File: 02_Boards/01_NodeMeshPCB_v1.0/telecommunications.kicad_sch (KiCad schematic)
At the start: 4 parts, among them J3 SMAJPHRATH1, U10 LC76GABMD, U5 HT-RA62

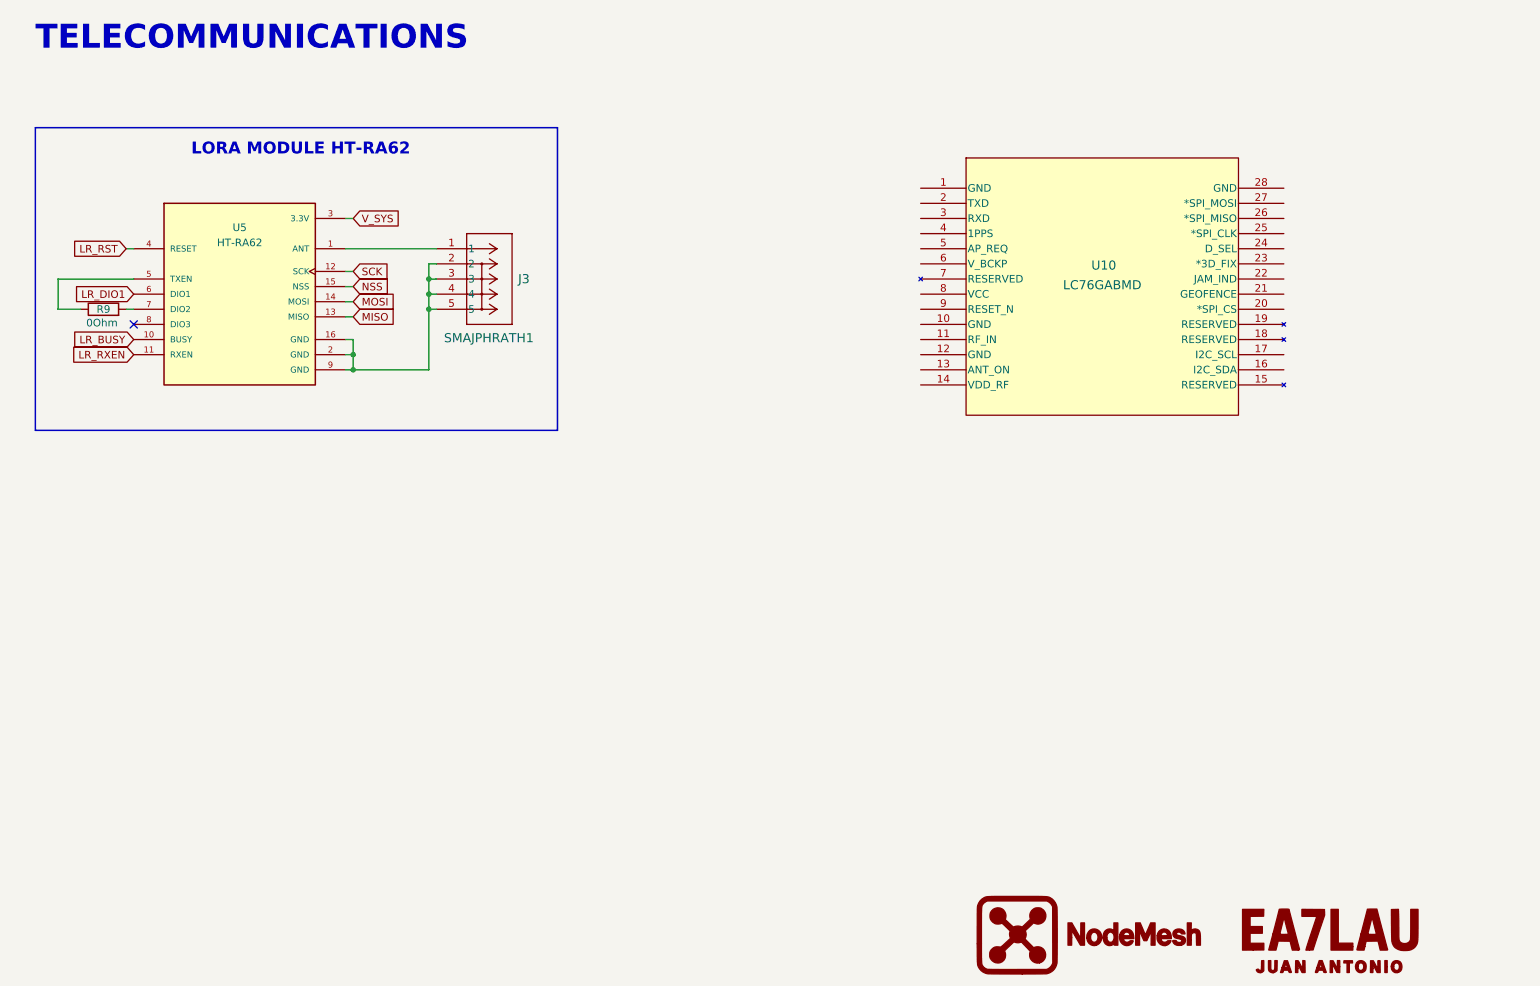
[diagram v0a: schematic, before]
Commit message: PCB placement
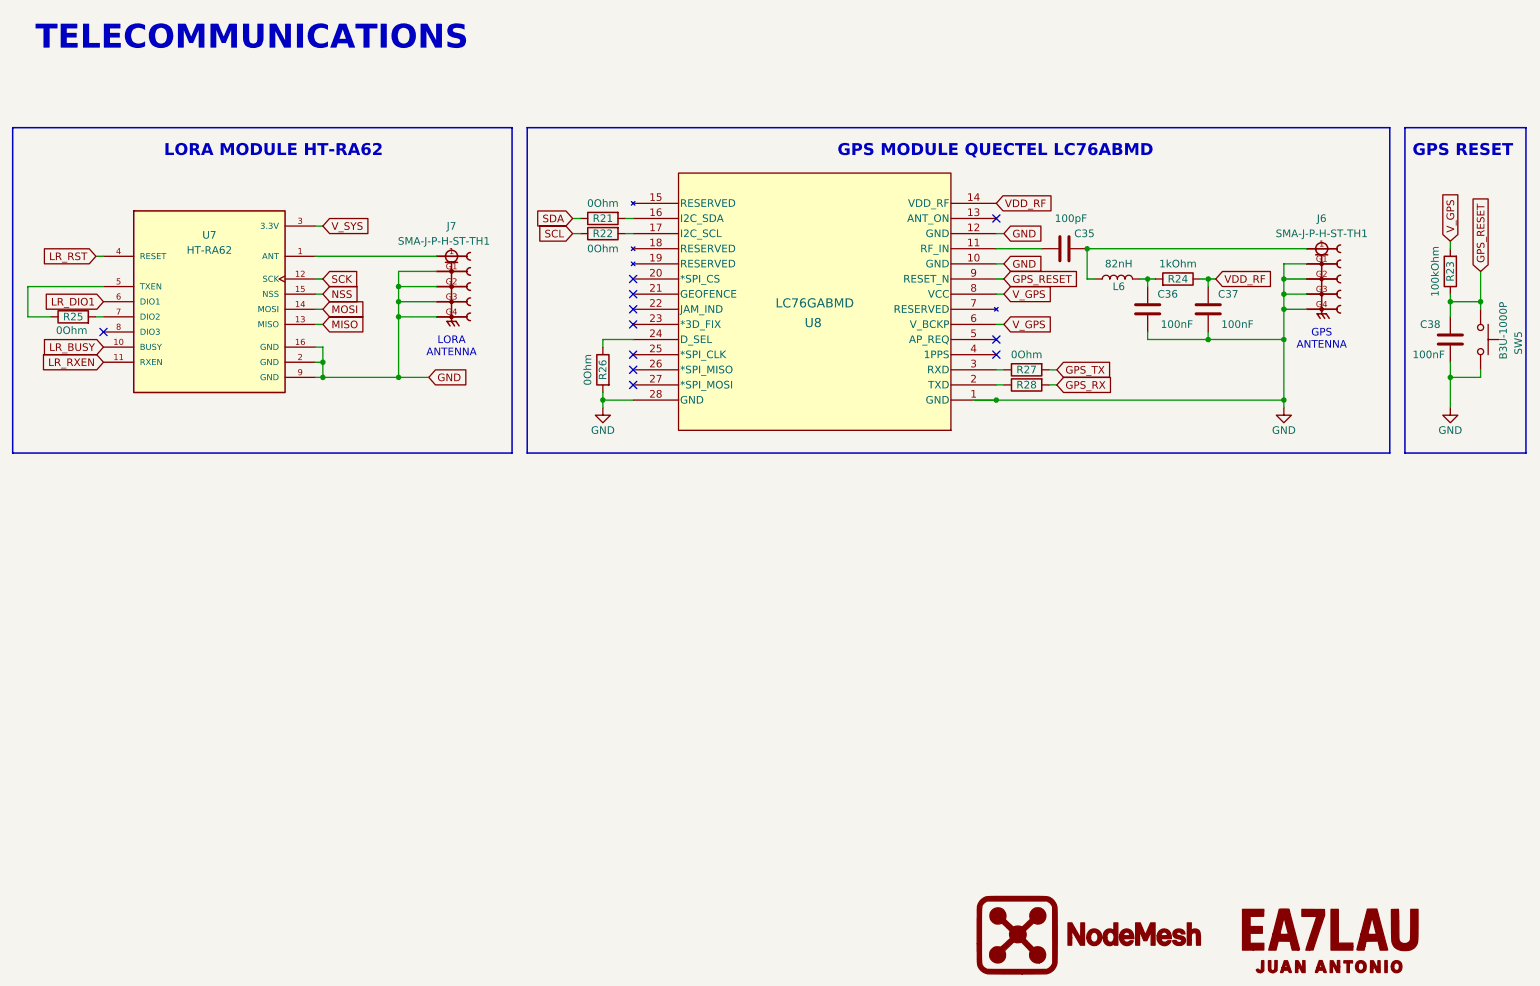
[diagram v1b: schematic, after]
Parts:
- removed J3: SMAJPHRATH1, CONN_SMA-J-P-H-RA-TH1_SAI, symbol SMAJPHRATH1:SMA-J-P-H-RA-TH1
- added C35: 100pF, Capacitor_SMD:C_0603_1608Metric, symbol Device:C
- added C36, C37, C38: 100nF, Capacitor_SMD:C_0603_1608Metric, symbol Device:C
- added J6, J7: SMA-J-P-H-ST-TH1, 01_Footprints:SMA-J-P-H-ST-TH1, symbol SMA-J-P-H-ST-TH1:SMA-J-P-H-ST-TH1
- added L6: 82nH, Inductor_SMD:L_0603_1608Metric, symbol Device:L
- added R21, R22, R26, R27, R28: 0Ohm, Resistor_SMD:R_0603_1608Metric, symbol Device:R
- added R23: 100kOhm, Resistor_SMD:R_0603_1608Metric, symbol Device:R
- added R24: 1kOhm, Resistor_SMD:R_0603_1608Metric, symbol Device:R
- added SW5: B3U-1000P, Button_Switch_SMD:SW_SPST_B3U-1000P, symbol Switch:SW_Push
- R25: renamed from R9; footprint (none) -> Resistor_SMD:R_0603_1608Metric
- U7: renamed from U5; footprint (none) -> 01_Footprints:HT-RA62
- U8: renamed from U10; footprint LC76G_QWS -> 01_Footprints:LC76GABMD
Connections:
- net GND: now reaches U8.1 (GND)
- net GND: now also U7.16 (GND), U7.2 (GND), U7.9 (GND), U8.10 (GND), U8.12 (GND), U8.28 (GND), C36.2, C37.2, C38.2, J6.G1, J6.G2, J6.G3, J6.G4, J7.G1, J7.G2, J7.G3, J7.G4, R26.2, SW5.2
- net at U8.11 (RF_IN): now also C35.1
- net VDD_RF: now reaches U8.14 (VDD_RF)
- net VDD_RF: now also C37.1, R24.1
- net at U8.16 (I2C_SDA): now also R21.2
- net at U8.17 (I2C_SCL): now also R22.2
- net at U8.2 (TXD): now also R28.1
- net at U8.24 (D_SEL): now also R26.1
- net at U8.3 (RXD): now also R27.1
- net V_GPS: now reaches U8.6 (V_BCKP)
- net V_GPS: now also U8.8 (VCC), R23.2
- net GPS_RESET: now reaches U8.9 (RESET_N)
- net GPS_RESET: now also C38.1, R23.1, SW5.1
- net at U7.1 (ANT): now also J7.1
- new net: C36.1, L6.1, R24.2
- new net: C35.2, J6.1, L6.2
- new net GPS_RX: R28.2
- new net GPS_TX: R27.2
- new net SCL: R22.1
- new net SDA: R21.1
- no-connect marks 1 -> 11
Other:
- note added: "GPS ANTENNA"
- note added: "GPS MODULE QUECTEL LC76ABMD"
- note added: "GPS RESET"
- note added: "LORA ANTENNA"
- moved on the sheet: R25, U7, U8
